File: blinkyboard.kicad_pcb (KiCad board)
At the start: 2 copper layers, 20 parts, among them J1 Conn_01x02_Socket, SW1 SW_Push, U1 NE555P, U2 4017

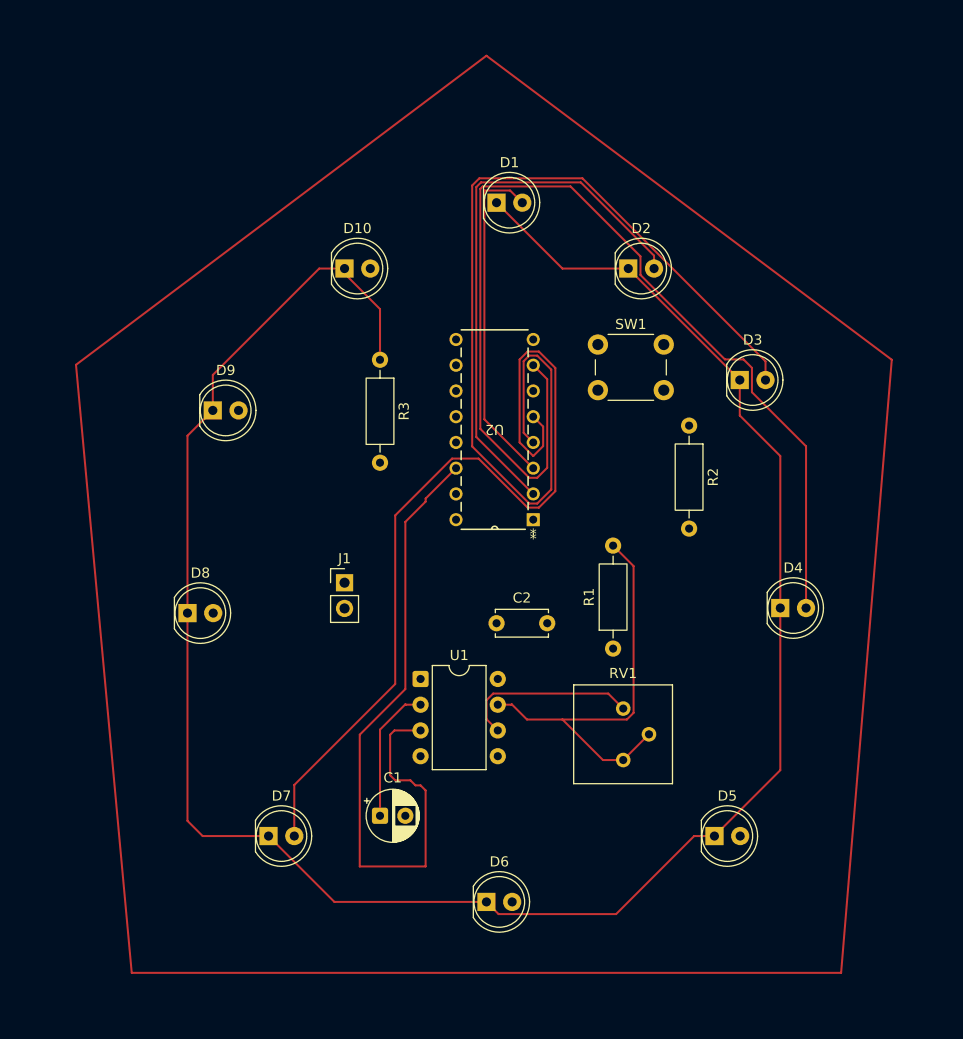
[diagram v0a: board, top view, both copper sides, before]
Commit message: Final update for KiCad files.
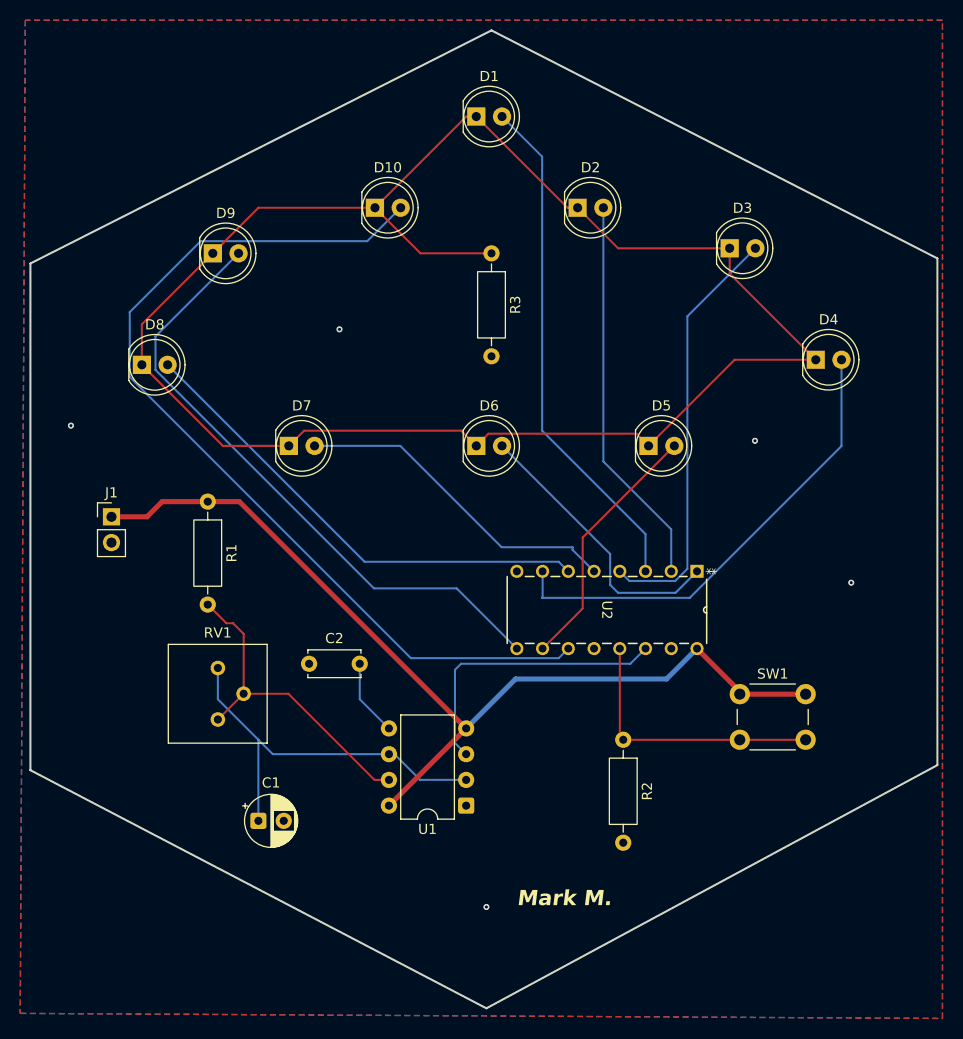
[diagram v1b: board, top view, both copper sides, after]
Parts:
- moved D6 45.0 mm to (149.0, 93.5)
- moved R1 42.5 mm to (122.5, 99.0), turned to -90 degrees
- moved RV1 40.2 mm to (123.5, 120.5)
- moved D5 39.0 mm to (166.0, 93.5)
- moved D7 38.6 mm to (130.5, 93.5)
- moved SW1 37.2 mm to (175.0, 118.0)
- moved R2 31.7 mm to (163.5, 122.5)
- moved U2 31.1 mm to (153.0, 113.5), turned to -90 degrees
- moved D8 24.9 mm to (116.0, 85.5)
- moved D4 24.7 mm to (182.5, 85.0)
- moved J1 23.9 mm to (113.0, 100.5)
- moved C2 18.9 mm to (132.5, 115.0)
- moved D9 15.5 mm to (123.0, 74.5)
- moved R3 15.2 mm to (150.5, 74.5)
- moved U1 13.3 mm to (148.0, 129.0), turned to 180 degrees
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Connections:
- J1 pad 1: unconnected-(J1-Pin_1-Pad1) -> +5V
- J1 pad 2: unconnected-(J1-Pin_2-Pad2) -> GND
- SW1 pad 1: unconnected-(SW1-Pad1) -> +5V
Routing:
- net +5V: track 0.00 -> 94.5 mm
- net Net-(D10-A): track 0.00 -> 92.6 mm
- net Net-(D9-A): track 0.00 -> 61.9 mm
- net Net-(D4-A): track 104.7 -> 46.9 mm
- net Net-(D3-A): track 98.8 -> 42.0 mm
- net Net-(D7-A): track 88.0 -> 32.9 mm
- net Net-(D8-A): track 0.00 -> 48.0 mm
- net OUT: track 68.5 -> 28.4 mm
- net Net-(D1-K): track 212.4 -> 179.8 mm
- net Net-(D6-A): track 0.00 -> 27.9 mm
- net Net-(U2-CKEN): track 0.00 -> 27.1 mm
- net Net-(D5-A): track 0.00 -> 25.4 mm
- net Net-(D1-A): track 33.6 -> 50.7 mm
- net Net-(D2-A): track 54.6 -> 38.7 mm
- net Net-(U1-DISCH): track 42.9 -> 32.1 mm
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- added copper zone on B.Cu, net GND
- added copper zone on F.Cu, net GND
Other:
- board outline added: 89.5 x 96.5 mm
- board text added: "Mark M."
